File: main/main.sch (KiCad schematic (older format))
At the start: 2 parts, among them J2 AudioJack3, J3 Conn_02x10_Odd_Even

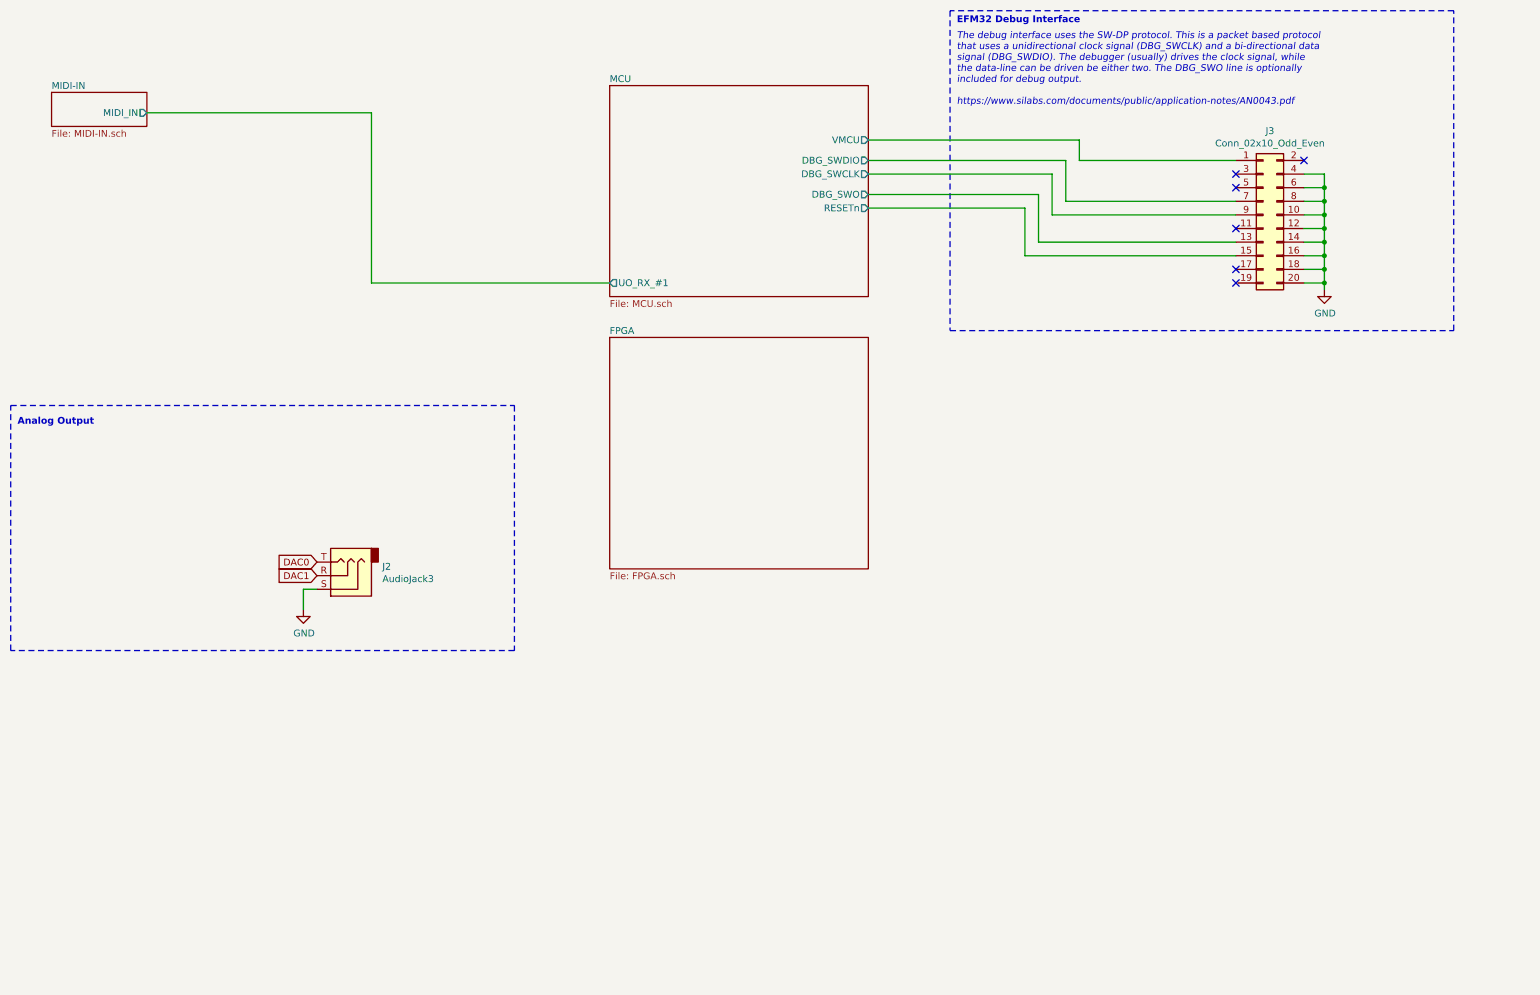
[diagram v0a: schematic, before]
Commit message: Some cleanup
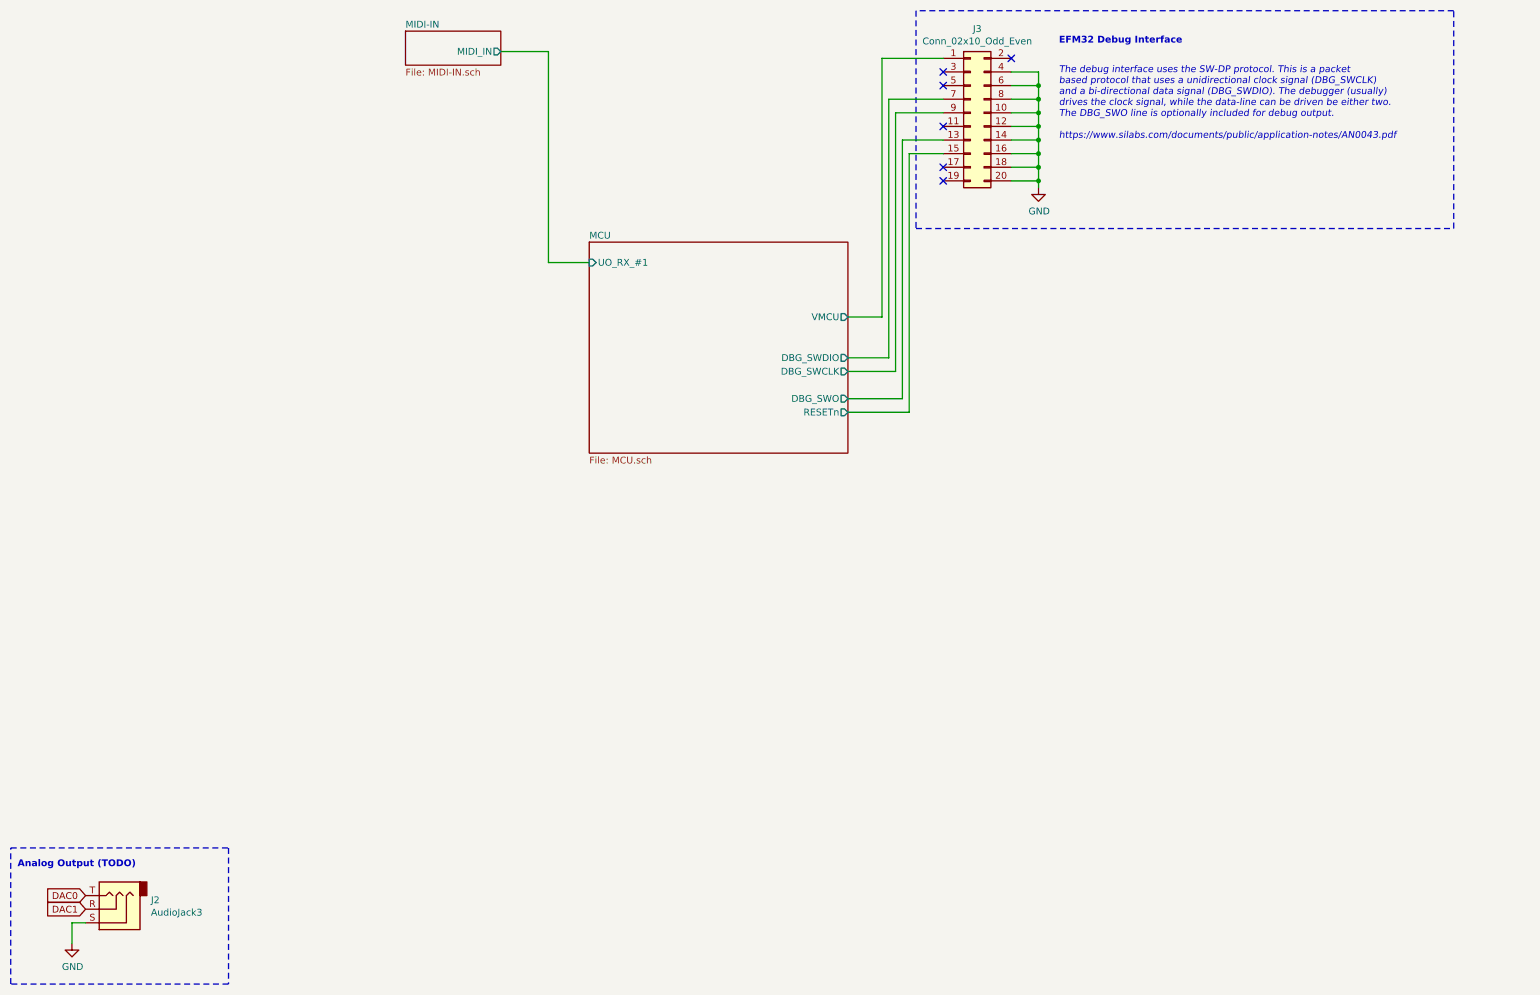
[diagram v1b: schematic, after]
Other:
- note added: "Analog Output (TODO)"
- note added: "The debug interface uses the SW-DP protocol. This is a packet \nbased protocol that uses a unidirectional clock signal (DBG_SWCLK) \nand a bi-directional data signal (DBG_SWDIO). The debugger (usually)\ndrives the clock signal, while the data-line can be driven be either two.\nThe DBG_SWO line is optionally included for debug output.\n\nhttps://www.silabs.com/documents/public/application-notes/AN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"
- note removed: "Analog Output"
- note removed: "The debug interface uses the SW-DP protocol. This is a packet based protocol\nthat uses a unidirectional clock signal (DBG_SWCLK) and a bi-directional data\nsignal (DBG_SWDIO). The debugger (usually) drives the clock signal, while\nthe data-line can be driven be either two. The DBG_SWO line is optionally\nincluded for debug output.\n\nhttps://www.silabs.com/documents/public/application-notes/AN00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"
- moved on the sheet: J2, J3
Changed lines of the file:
@@
 $Descr A4 11693 8268
 encoding utf-8
-Sheet 1 4
+Sheet 1 3
 Title "Synthesizer"
 Date "2021-09-06"
@@
 L Connector:AudioJack3 J2
 U 1 1 61366BDF
-P 3000 4700
-F 0 "J2" H 2720 4633 50  0000 R CNN
-F 1 "AudioJack3" H 2720 4724 50  0000 R CNN
-F 2 "" H 3000 4700 50  0001 C CNN
-F 3 "~" H 3000 4700 50  0001 C CNN
-	1    3000 4700
+P 1300 7150
+F 0 "J2" H 1020 7083 50  0000 R CNN
+F 1 "AudioJack3" H 1020 7174 50  0000 R CNN
+F 2 "" H 1300 7150 50  0001 C CNN
+F 3 "~" H 1300 7150 50  0001 C CNN
+	1    1300 7150
 	-1   0    0    1
 $EndComp
@@
 L power:GND #PWR0101
 U 1 1 61367C82
-P 2700 4950
-F 0 "#PWR0101" H 2700 4700 50  0001 C CNN
-F 1 "GND" H 2705 4777 50  0000 C CNN
-F 2 "" H 2700 4950 50  0001 C CNN
-F 3 "" H 2700 4950 50  0001 C CNN
-	1    2700 4950
+P 1000 7400
+F 0 "#PWR0101" H 1000 7150 50  0001 C CNN
+F 1 "GND" H 1005 7227 50  0000 C CNN
+F 2 "" H 1000 7400 50  0001 C CNN
+F 3 "" H 1000 7400 50  0001 C CNN
+	1    1000 7400
 	1    0    0    -1
 $EndComp
 Wire Wire Line
-	2700 4950 2700 4800
+	1000 7400 1000 7250
 Wire Wire Line
-	2700 4800 2800 4800
-Text GLabel 2800 4600 0    50   Input ~ 0
+	1000 7250 1100 7250
+Text GLabel 1100 7050 0    50   Input ~ 0
 DAC0
-Text GLabel 2800 4700 0    50   Input ~ 0
+Text GLabel 1100 7150 0    50   Input ~ 0
 DAC1
 Wire Notes Line
-	550  3450 4250 3450
+	550  6700 2150 6700
 Wire Notes Line
-	4250 5250 550  5250
-Text Notes 600  3600 0    50   ~ 10
-Analog Output
+	2150 7700 550  7700
+Text Notes 600  6850 0    50   ~ 10
+Analog Output (TODO)
 Wire Notes Line
-	4250 3450 4250 5250
+	2150 6700 2150 7700
 Wire Notes Line
-	550  5250 550  3450
+	550  7700 550  6700
 Wire Notes Line
-	7450 2900 11150 2900
-Wire Notes Line
-	11150 2900 11150 550
-Wire Notes Line
-	11150 550  7450 550
-Wire Notes Line
-	7450 550  7450 2900
-Text Notes 7500 650  0    50   ~ 10
-EFM32 Debug Interface
+	11150 550  7200 550
+$Sheet
+S 4800 2250 1900 1550
+U 6139E7E0
+F0 "MCU" 50
+F1 "MCU.sch" 50
+F2 "DBG_SWDIO" O R 6700 3100 50
+F3 "DBG_SWCLK" O R 6700 3200 50
+F4 "DBG_SWO" O R 6700 3400 50
+F5 "RESETn" O R 6700 3500 50
+F6 "VMCU" O R 6700 2800 50
+F7 "UO_RX_#1" I L 4800 2400 50
+$EndSheet
+$Sheet
+S 3450 700  700  250
+U 613F97F2
+F0 "MIDI-IN" 50
+F1 "MIDI-IN.sch" 50
+F2 "MIDI_IN" O R 4150 850 50
+$EndSheet
+Text Notes 8250 1500 0    50   Italic 0
+The debug interface uses the SW-DP protocol. This is a packet \nbased protocol that uses a unidirectional clock signal (DBG_SWCLK) \nand a bi-directional data signal (DBG_SWDIO). The debugger (usually)\ndrives the clock signal, while the data-line can be driven be either two.\nThe DBG_SWO line is optionally included for debug output.\n\nhttps://www.silabs.com/documents/public/application-notes/AN0043.pdf
+NoConn ~ 7400 1800
+NoConn ~ 7400 1700
+Wire Wire Line
+	8100 1100 8100 1200
+Connection ~ 8100 1100
+Wire Wire Line
+	8100 1000 8100 1100
+Wire Wire Line
+	7900 1000 8100 1000
+Connection ~ 8100 1200
+Wire Wire Line
+	7900 1100 8100 1100
+Wire Wire Line
+	8100 1300 8100 1400
+Connection ~ 8100 1300
+Wire Wire Line
+	8100 1200 8100 1300
+Wire Wire Line
+	7900 1200 8100 1200
+Connection ~ 8100 1400
+Wire Wire Line
+	7900 1300 8100 1300
+Wire Wire Line
+	8100 1500 8100 1600
+Connection ~ 8100 1500
+Wire Wire Line
+	8100 1400 8100 1500
+Wire Wire Line
+	7900 1400 8100 1400
+Wire Wire Line
+	8100 1600 8100 1700
+Connection ~ 8100 1600
+Wire Wire Line
+	7900 1500 8100 1500
+Connection ~ 8100 1700
+Wire Wire Line
+	7900 1600 8100 1600
+Wire Wire Line
+	8100 1800 8100 1850
+Connection ~ 8100 1800
+Wire Wire Line
+	8100 1700 8100 1800
+Wire Wire Line
+	7900 1700 8100 1700
+Wire Wire Line
+	7900 1800 8100 1800
+$Comp
+L power:GND #PWR04
+U 1 1 613B8CA5
+P 8100 1850
+F 0 "#PWR04" H 8100 1600 50  0001 C CNN
+F 1 "GND" H 8105 1677 50  0000 C CNN
+F 2 "" H 8100 1850 50  0001 C CNN
+F 3 "" H 8100 1850 50  0001 C CNN
+	1    8100 1850
+	1    0    0    -1
+$EndComp
+NoConn ~ 7400 1400
+NoConn ~ 7400 1100
+NoConn ~ 7400 1000
+NoConn ~ 7900 900
 $Comp
 L Connector_Generic:Conn_02x10_Odd_Even J3
 U 1 1 613A6A76
-P 9750 2050
-F 0 "J3" H 9800 2667 50  0000 C CNN
-F 1 "Conn_02x10_Odd_Even" H 9800 2576 50  0000 C CNN
-F 2 "" H 9750 2050 50  0001 C CNN
-F 3 "~" H 9750 2050 50  0001 C CNN
-	1    9750 2050
+P 7600 1300
+F 0 "J3" H 7650 1917 50  0000 C CNN
+F 1 "Conn_02x10_Odd_Even" H 7650 1826 50  0000 C CNN
+F 2 "" H 7600 1300 50  0001 C CNN
+F 3 "~" H 7600 1300 50  0001 C CNN
+	1    7600 1300
 	1    0    0    -1
 $EndComp
-NoConn ~ 10050 1650
-NoConn ~ 9550 1750
-NoConn ~ 9550 1850
-NoConn ~ 9550 2150
-$Comp
-L power:GND #PWR04
-U 1 1 613B8CA5
-P 10200 2600
-F 0 "#PWR04" H 10200 2350 50  0001 C CNN
-F 1 "GND" H 10205 2427 50  0000 C CNN
-F 2 "" H 10200 2600 50  0001 C CNN
-F 3 "" H 10200 2600 50  0001 C CNN
-	1    10200 2600
-	1    0    0    -1
-$EndComp
+Text Notes 8250 800  0    50   ~ 10
+EFM32 Debug Interface
+Wire Notes Line
+	7200 550  7200 2150
+Wire Notes Line
+	11150 2150 11150 550
+Wire Notes Line
+	7200 2150 11150 2150
 Wire Wire Line
-	10050 2550 10200 2550
+	6700 2800 6950 2800
 Wire Wire Line
-	10050 2450 10200 2450
+	6950 2800 6950 900
 Wire Wire Line
-	10200 2450 10200 2550
-Connection ~ 10200 2550
+	6950 900  7400 900
 Wire Wire Line
-	10200 2550 10200 2600
+	6700 3100 7000 3100
 Wire Wire Line
-	10050 2350 10200 2350
-Connection ~ 10200 2450
+	7000 3100 7000 1200
 Wire Wire Line
-	10050 2250 10200 2250
-Connection ~ 10200 2350
+	7000 1200 7400 1200
 Wire Wire Line
-	10200 2350 10200 2450
+	6700 3200 7050 3200
 Wire Wire Line
-	10050 2150 10200 2150
+	7050 3200 7050 1300
 Wire Wire Line
-	10200 2150 10200 2250
-Connection ~ 10200 2250
+	7050 1300 7400 1300
 Wire Wire Line
-	10200 2250 10200 2350
+	6700 3400 7100 3400
 Wire Wire Line
-	10050 2050 10200 2050
-Connection ~ 10200 2150
+	7100 3400 7100 1500
 Wire Wire Line
-	10050 1950 10200 1950
+	7100 1500 7400 1500
 Wire Wire Line
-	10200 1950 10200 2050
-Connection ~ 10200 2050
+	6700 3500 7150 3500
 Wire Wire Line
-	10200 2050 10200 2150
+	7150 3500 7150 1600
 Wire Wire Line
-	10050 1850 10200 1850
-Connection ~ 10200 1950
+	7150 1600 7400 1600
 Wire Wire Line
-	10050 1750 10200 1750
+	4150 850  4500 850
 Wire Wire Line
-	10200 1750 10200 1850
-Connection ~ 10200 1850
+	4500 850  4500 2400
 Wire Wire Line
-	10200 1850 10200 1950
-NoConn ~ 9550 2450
-NoConn ~ 9550 2550
-Text Notes 7500 1250 0    50   Italic 0
-The debug interface uses the SW-DP protocol. This is a packet based protocol\nthat uses a unidirectional clock signal (DBG_SWCLK) and a bi-directional data\nsignal (DBG_SWDIO). The debugger (usually) drives the clock signal, while\nthe data-line can be driven be either two. The DBG_SWO line is optionally\nincluded for debug output.\n\nhttps://www.silabs.com/documents/public/application-notes/AN0043.pdf
-$Sheet
-S 4950 2950 1900 1700
-U 6139EB2D
-F0 "FPGA" 50
-F1 "FPGA.sch" 50
-$EndSheet
-Wire Wire Line
-	9550 2350 8000 2350
-Wire Wire Line
-	8000 2350 8000 2000
-Wire Wire Line
-	8000 2000 6850 2000
-Wire Wire Line
-	9550 2250 8100 2250
-Wire Wire Line
-	8100 2250 8100 1900
-Wire Wire Line
-	8100 1900 6850 1900
-Wire Wire Line
-	9550 2050 8200 2050
-Wire Wire Line
-	8200 2050 8200 1750
-Wire Wire Line
-	8200 1750 6850 1750
-Wire Wire Line
-	9550 1950 8300 1950
-Wire Wire Line
-	8300 1950 8300 1650
-Wire Wire Line
-	8300 1650 6850 1650
-Wire Wire Line
-	9550 1650 8400 1650
-Wire Wire Line
-	8400 1650 8400 1500
-Wire Wire Line
-	8400 1500 6850 1500
-$Sheet
-S 4950 1100 1900 1550
-U 6139E7E0
-F0 "MCU" 50
-F1 "MCU.sch" 50
-F2 "DBG_SWDIO" O R 6850 1650 50
-F3 "DBG_SWCLK" O R 6850 1750 50
-F4 "DBG_SWO" O R 6850 1900 50
-F5 "RESETn" O R 6850 2000 50
-F6 "VMCU" O R 6850 1500 50
-F7 "UO_RX_#1" O L 4950 2550 50
-$EndSheet
-$Sheet
-S 850  1150 700  250
-U 613F97F2
-F0 "MIDI-IN" 50
-F1 "MIDI-IN.sch" 50
-F2 "MIDI_IN" O R 1550 1300 50
-$EndSheet
-Wire Wire Line
-	1550 1300 3200 1300
-Wire Wire Line
-	3200 1300 3200 2550
-Wire Wire Line
-	3200 2550 4950 2550
+	4500 2400 4800 2400
 $EndSCHEMATC
